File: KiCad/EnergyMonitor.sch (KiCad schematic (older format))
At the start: 70 parts, among them J1 Conn_01x04, J10 AudioJack3_Ground_Switch_5_pin, J11 Conn_01x02, J13 Barrel_Jack_Switch, J14 Conn_01x04, J15 Conn_01x04, J16 4P4C, J2 Conn_01x04, J3 Conn_01x04, J4 Conn_01x04, J5 Conn_01x04, J6 Conn_01x04, J7 Conn_01x02, J8 AudioJack3_Ground_Switch_5_pin, J9 AudioJack3_Ground_Switch_5_pin, U1 ESP32_D1_MINI, U2 HT7333

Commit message: circuit design & pcb layout
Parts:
- R14: footprint LED_SMD:LED_0805_2012Metric -> Resistor_SMD:R_0805_2012Metric
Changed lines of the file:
@@
 F 0 "R14" H 5595 6896 50  0000 L CNN
 F 1 "4K7" H 5595 6805 50  0000 L CNN
-F 2 "LED_SMD:LED_0805_2012Metric" V 5455 6850 50  0001 C CNN
+F 2 "Resistor_SMD:R_0805_2012Metric" V 5455 6850 50  0001 C CNN
 F 3 "~" H 5525 6850 50  0001 C CNN
 	1    5525 6850

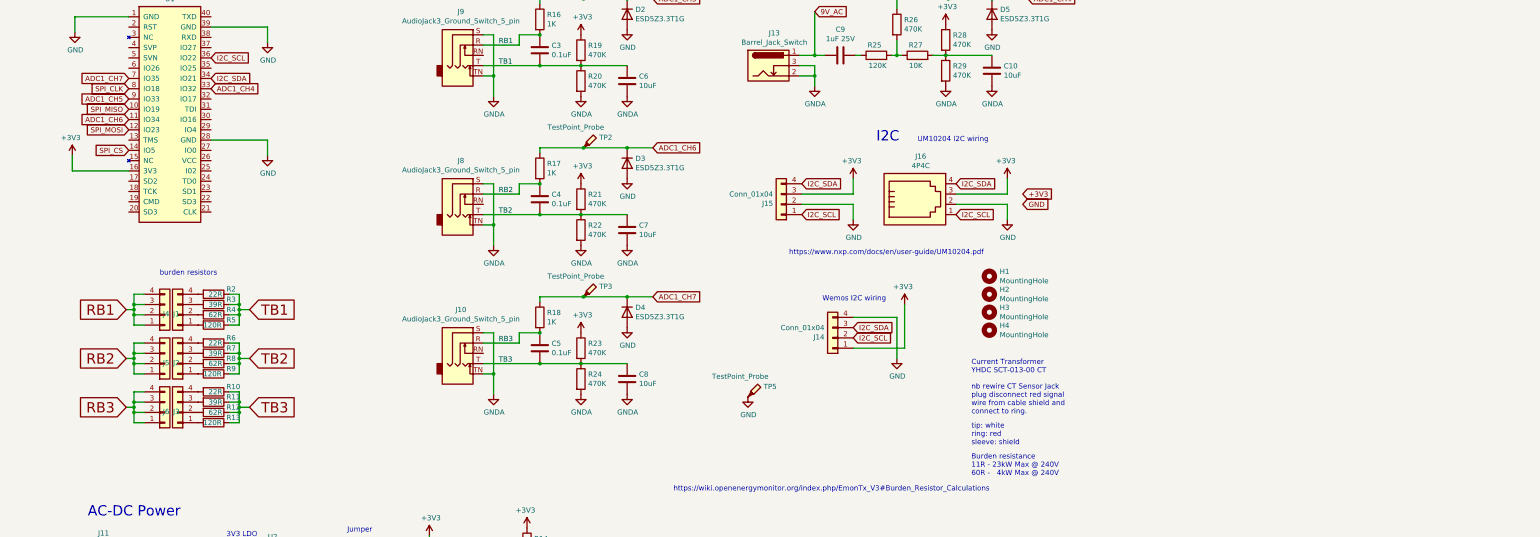
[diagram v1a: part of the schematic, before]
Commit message: circuit design & pcb layout
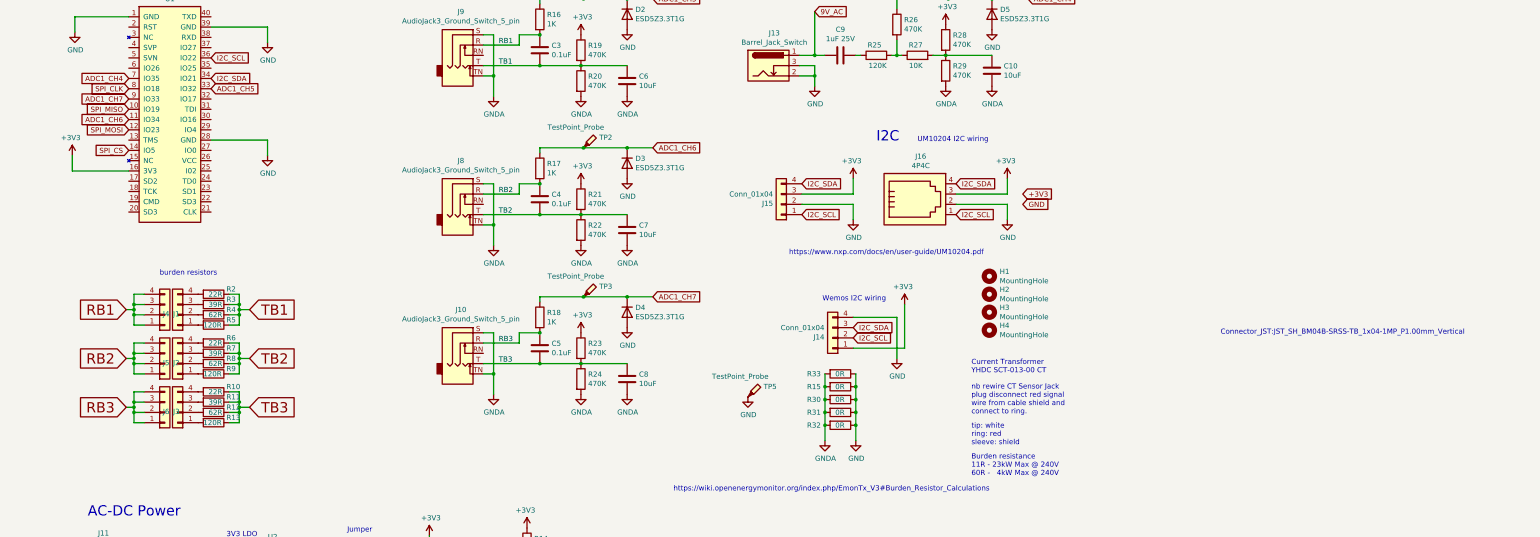
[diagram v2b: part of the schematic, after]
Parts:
- added R15, R30, R31, R32, R33: 0R, Resistor_SMD:R_0805_2012Metric, symbol Device:R
- J14: footprint Connector_JST:JST_SH_SM04B-SRSS-TB_1x04-1MP_P1.00mm_Horizontal -> Connector_JST:JST_SH_BM04B-SRSS-TB_1x04-1MP_P1.00mm_Vertical
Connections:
- net ADC1_CH4: now also U1.7 (IO35); no longer U1.33 (IO32)
- net ADC1_CH5: now also U1.33 (IO32); no longer U1.9 (IO33)
- net ADC1_CH7: now also U1.9 (IO33); no longer U1.7 (IO35)
- net GND: now also J13.2, J13.3, R15.1, R30.1, R31.1, R32.1, R33.1
- net GNDA: now also R15.2, R30.2, R31.2, R32.2, R33.2; no longer J13.2, J13.3
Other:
- note added: "Connector_JST:JST_SH_BM04B-SRSS-TB_1x04-1MP_P1.00mm_Vertical"
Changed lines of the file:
@@
 Sheet 1 1
 Title "ESP32 Energy Monitor"
-Date "2021-09-22"
+Date "2021-09-24"
 Rev "v1.0"
 Comp ""
@@
 Text GLabel 1650 2725 0    50   Input ~ 0
 ADC1_CH6
-Text GLabel 1650 2325 0    50   Input ~ 0
+Text GLabel 1650 2525 0    50   Input ~ 0
 ADC1_CH7
 Text Notes 9850 5200 0    50   ~ 0
@@
 	1    0    0    -1
 $EndComp
-$Comp
-L power:GNDA #PWR024
-U 1 1 613562F0
-P 8325 2400
-F 0 "#PWR024" H 8325 2150 50  0001 C CNN
-F 1 "GNDA" H 8330 2227 50  0000 C CNN
-F 2 "" H 8325 2400 50  0001 C CNN
-F 3 "" H 8325 2400 50  0001 C CNN
-	1    8325 2400
-	1    0    0    -1
-$EndComp
 Wire Wire Line
 	8175 2300 8325 2300
@@
 Text Notes 4000 7550 0    50   ~ 0
 Remove Jumper\nif ESP32 powered\nby USB.
-Text GLabel 1650 2525 0    50   Input ~ 0
-ADC1_CH5
 Text GLabel 2450 2425 2    50   Input ~ 0
+ADC1_CH5
+Text GLabel 1650 2325 0    50   Input ~ 0
 ADC1_CH4
 Text GLabel 2450 2125 2    50   Input ~ 0
@@
 F 0 "J14" H 8580 4842 50  0000 L CNN
 F 1 "Conn_01x04" H 8580 4751 50  0000 L CNN
-F 2 "Connector_JST:JST_SH_SM04B-SRSS-TB_1x04-1MP_P1.00mm_Horizontal" H 8500 4850 50  0001 C CNN
+F 2 "Connector_JST:JST_SH_BM04B-SRSS-TB_1x04-1MP_P1.00mm_Vertical" H 8500 4850 50  0001 C CNN
 F 3 "~" H 8500 4850 50  0001 C CNN
 	1    8500 4850
@@
 Text Notes 5875 7425 0    50   ~ 0
 red superbright LED\n0805 SMD\ngreen band -ve\n1k R => 1.4mA\n4K7 => 0.3mA\n@3.3v
+$Comp
+L power:GND #PWR0106
+U 1 1 6153C70C
+P 8325 2400
+F 0 "#PWR0106" H 8325 2150 50  0001 C CNN
+F 1 "GND" H 8330 2227 50  0000 C CNN
+F 2 "" H 8325 2400 50  0001 C CNN
+F 3 "" H 8325 2400 50  0001 C CNN
+	1    8325 2400
+	1    0    0    -1
+$EndComp
+$Comp
+L power:GND #PWR0107
+U 1 1 61546152
+P 8725 5850
+F 0 "#PWR0107" H 8725 5600 50  0001 C CNN
+F 1 "GND" H 8730 5677 50  0000 C CNN
+F 2 "" H 8725 5850 50  0001 C CNN
+F 3 "" H 8725 5850 50  0001 C CNN
+	1    8725 5850
+	1    0    0    -1
+$EndComp
+$Comp
+L power:GNDA #PWR0108
+U 1 1 61546DE3
+P 8425 5850
+F 0 "#PWR0108" H 8425 5600 50  0001 C CNN
+F 1 "GNDA" H 8430 5677 50  0000 C CNN
+F 2 "" H 8425 5850 50  0001 C CNN
+F 3 "" H 8425 5850 50  0001 C CNN
+	1    8425 5850
+	1    0    0    -1
+$EndComp
+Text Notes 12275 4825 0    50   ~ 0
+Connector_JST:JST_SH_BM04B-SRSS-TB_1x04-1MP_P1.00mm_Vertical
+$Comp
+L Device:R R32
+U 1 1 6154DEF5
+P 8575 5700
+F 0 "R32" V 8575 5375 50  0000 L CNN
+F 1 "0R" V 8575 5650 50  0000 L CNN
+F 2 "Resistor_SMD:R_0805_2012Metric" V 8505 5700 50  0001 C CNN
+F 3 "~" H 8575 5700 50  0001 C CNN
+	1    8575 5700
+	0    1    1    0
+$EndComp
+$Comp
+L Device:R R31
+U 1 1 6154EEF3
+P 8575 5575
+F 0 "R31" V 8575 5250 50  0000 L CNN
+F 1 "0R" V 8575 5525 50  0000 L CNN
+F 2 "Resistor_SMD:R_0805_2012Metric" V 8505 5575 50  0001 C CNN
+F 3 "~" H 8575 5575 50  0001 C CNN
+	1    8575 5575
+	0    1    1    0
+$EndComp
+$Comp
+L Device:R R30
+U 1 1 615542A9
+P 8575 5450
+F 0 "R30" V 8575 5125 50  0000 L CNN
+F 1 "0R" V 8575 5400 50  0000 L CNN
+F 2 "Resistor_SMD:R_0805_2012Metric" V 8505 5450 50  0001 C CNN
+F 3 "~" H 8575 5450 50  0001 C CNN
+	1    8575 5450
+	0    1    1    0
+$EndComp
+$Comp
+L Device:R R15
+U 1 1 61554A8F
+P 8575 5325
+F 0 "R15" V 8575 5000 50  0000 L CNN
+F 1 "0R" V 8575 5275 50  0000 L CNN
+F 2 "Resistor_SMD:R_0805_2012Metric" V 8505 5325 50  0001 C CNN
+F 3 "~" H 8575 5325 50  0001 C CNN
+	1    8575 5325
+	0    1    1    0
+$EndComp
+Wire Wire Line
+	8725 5325 8725 5450
+Wire Wire Line
+	8725 5450 8725 5575
+Connection ~ 8725 5450
+Wire Wire Line
+	8725 5575 8725 5700
+Connection ~ 8725 5575
+Wire Wire Line
+	8725 5700 8725 5850
+Connection ~ 8725 5700
+Wire Wire Line
+	8425 5850 8425 5700
+Wire Wire Line
+	8425 5700 8425 5575
+Connection ~ 8425 5700
+Wire Wire Line
+	8425 5575 8425 5450
+Connection ~ 8425 5575
+Wire Wire Line
+	8425 5450 8425 5325
+Connection ~ 8425 5450
+$Comp
+L Device:R R33
+U 1 1 615B1549
+P 8575 5200
+F 0 "R33" V 8575 4875 50  0000 L CNN
+F 1 "0R" V 8575 5150 50  0000 L CNN
+F 2 "Resistor_SMD:R_0805_2012Metric" V 8505 5200 50  0001 C CNN
+F 3 "~" H 8575 5200 50  0001 C CNN
+	1    8575 5200
+	0    1    1    0
+$EndComp
+Wire Wire Line
+	8725 5200 8725 5325
+Connection ~ 8725 5325
+Wire Wire Line
+	8425 5200 8425 5325
+Connection ~ 8425 5325
 $EndSCHEMATC
